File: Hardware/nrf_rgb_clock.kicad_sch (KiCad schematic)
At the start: 49 parts, among them J1 Conn_01x02, J3 Conn_01x07_Pin, U1 AMS1117-3.3, U3 TPS54260DGQ, Y1 32MHz

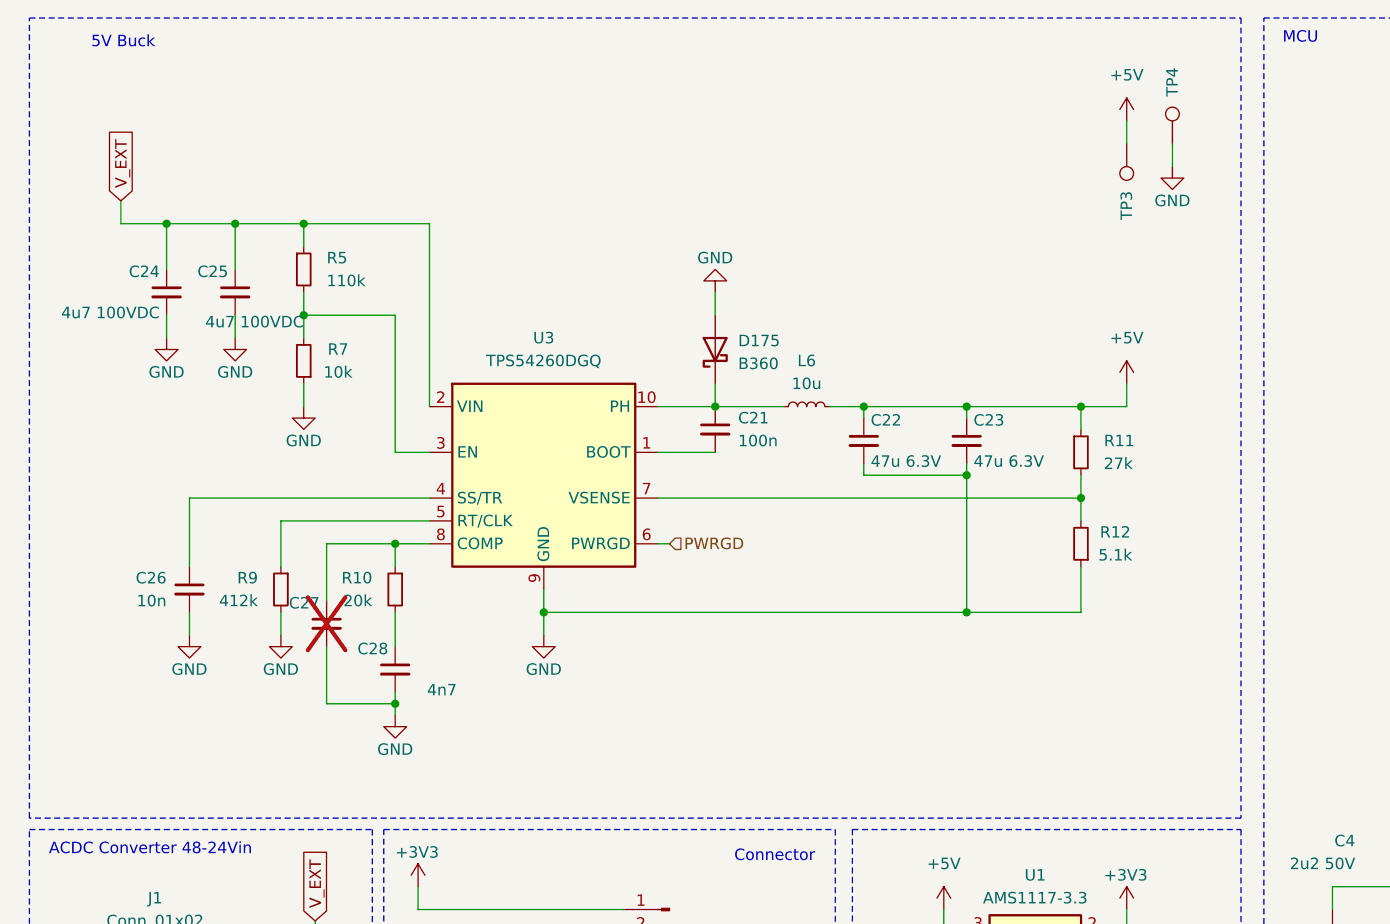
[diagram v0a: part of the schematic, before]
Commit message: new tps
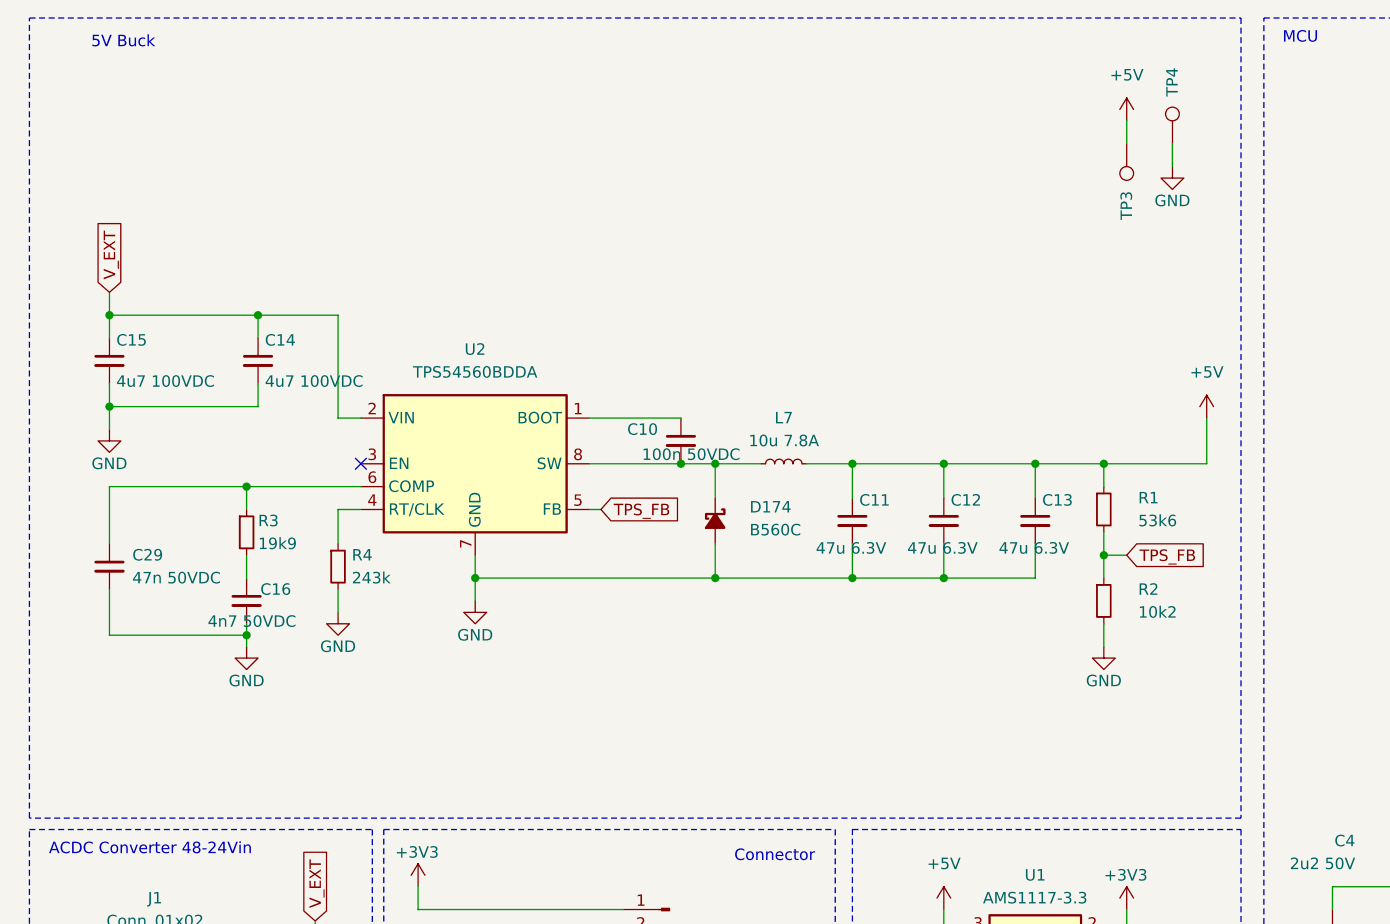
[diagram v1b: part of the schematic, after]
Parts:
- removed C21: 100n, Capacitor_SMD:C_0402_1005Metric, symbol Device:C_Small
- removed C22, C23: 47u 6.3V, Capacitor_SMD:C_0805_2012Metric, symbol Device:C_Small
- removed C24, C25: 4u7 100VDC, Capacitor_SMD:C_1206_3216Metric, symbol Device:C_Small
- removed C26: 10n, Capacitor_SMD:C_0402_1005Metric, symbol Device:C_Small
- removed C27: ~, Capacitor_SMD:C_0603_1608Metric, symbol Device:C_Small
- removed C28: 4n7, Capacitor_SMD:C_0603_1608Metric, symbol Device:C_Small
- removed D175: B360, Diode_SMD:D_SMC, symbol Diode:B360
- removed L6: 10u, ProjectFootprints:NRS5040T3R3NMGJV, symbol Device:L_Small
- removed R10: 20k, Resistor_SMD:R_0805_2012Metric, symbol Device:R_Small
- removed R11: 27k, Resistor_SMD:R_0805_2012Metric, symbol Device:R_Small
- removed R12: 5.1k, Resistor_SMD:R_0402_1005Metric, symbol Device:R_Small
- removed R5: 110k, Resistor_SMD:R_0805_2012Metric, symbol Device:R_Small
- removed R7: 10k, Resistor_SMD:R_0402_1005Metric, symbol Device:R_Small
- removed R9: 412k, Resistor_SMD:R_0805_2012Metric, symbol Device:R_Small
- removed U3: TPS54260DGQ, Package_SO:MSOP-10-1EP_3x3mm_P0.5mm_EP2.2x3.1mm_Mask1.83x1.89mm_ThermalVias, symbol Regulator_Switching:TPS54260DGQ
- added C10: 100n 50VDC, Capacitor_SMD:C_0805_2012Metric, symbol Device:C_Small
- added C11, C12, C13: 47u 6.3V, Capacitor_SMD:C_0805_2012Metric, symbol Device:C_Small
- added C14, C15: 4u7 100VDC, Capacitor_SMD:C_1206_3216Metric, symbol Device:C_Small
- added C16: 4n7 50VDC, Capacitor_SMD:C_0805_2012Metric, symbol Device:C_Small
- added C29: 47n 50VDC, Capacitor_SMD:C_0805_2012Metric, symbol Device:C_Small
- added D174: B560C, Diode_SMD:D_SMC, symbol Device:D_Schottky_Small_Filled
- added L7: 10u 7.8A, Inductor_SMD:L_Sunlord_MWSA1003S, symbol Device:L_Small
- added R1: 53k6, Resistor_SMD:R_0805_2012Metric, symbol Device:R_Small
- added R2: 10k2, Resistor_SMD:R_0805_2012Metric, symbol Device:R_Small
- added R3: 19k9, Resistor_SMD:R_0805_2012Metric, symbol Device:R_Small
- added R4: 243k, Resistor_SMD:R_0805_2012Metric, symbol Device:R_Small
- added U2: TPS54560BDDA, Package_SO:Texas_R-PDSO-G8_EP2.95x4.9mm_Mask2.4x3.1mm_ThermalVias, symbol Regulator_Switching:TPS54560BDDA
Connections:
- net +5V: now also C11.1, C12.1, C13.1, L7.2, R1.1
- net GND: now also C11.2, C12.2, C13.2, C14.2, C15.2, C16.2, C29.2, D174.2 (A), R2.2, R4.2, U2.7 (GND), U2.9 (GND)
- net V_EXT: now also C14.1, C15.1, U2.2 (VIN)
- new net: C10.2, D174.1 (K), L7.1, U2.8 (SW)
- new net: R4.1, U2.4 (RT/CLK)
- new net: C10.1, U2.1 (BOOT)
- new net: C16.1, R3.2
- new net: C29.1, R3.1, U2.6 (COMP)
- new net TPS_FB: R1.2, R2.1, U2.5 (FB)
- no-connect marks 3 -> 4
